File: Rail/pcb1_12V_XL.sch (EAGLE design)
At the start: 114 parts, among them J1 638207222006, J10 638207222006, J11 638207222006, J12 638207222006, J2 638207222006, U1 ESP32-S3-DEVKITC-1-N8R2, U4 TLE9250VSJ, X2 B4P-VH

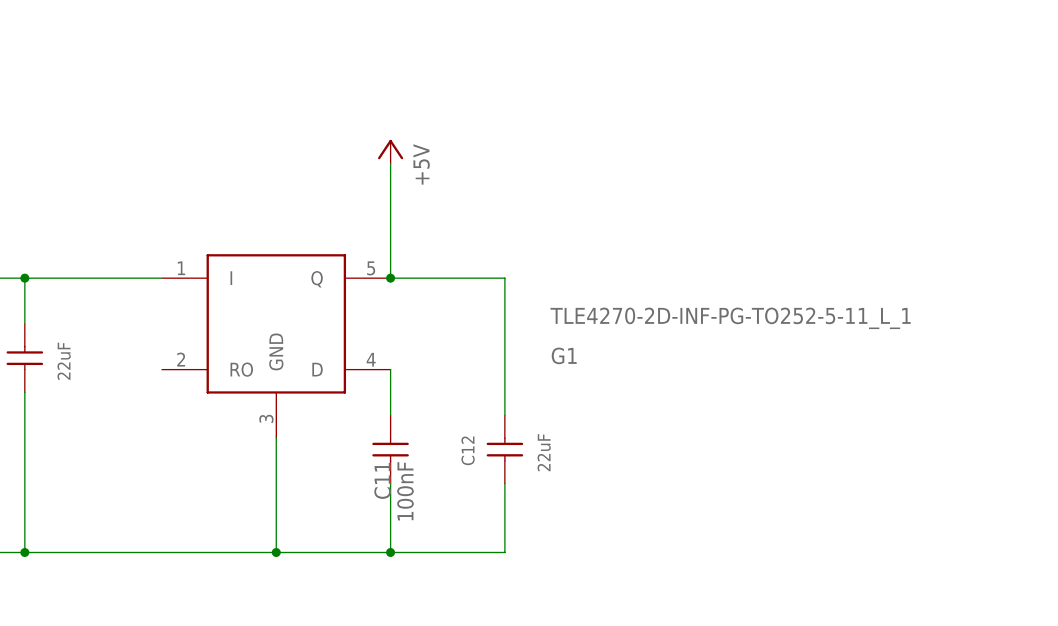
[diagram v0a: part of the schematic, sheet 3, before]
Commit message: Prepare Prouction
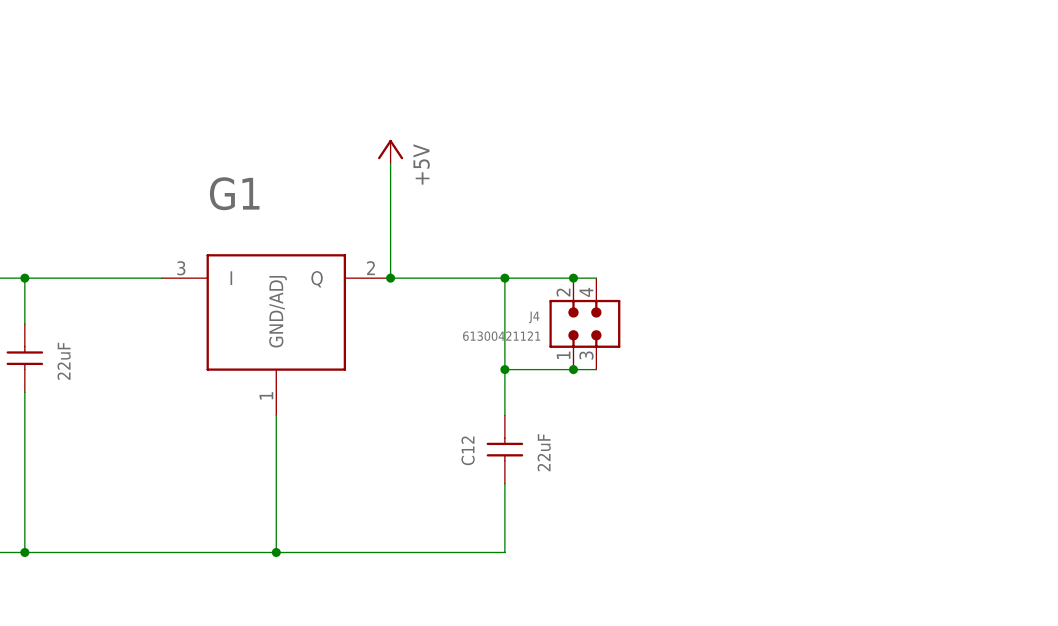
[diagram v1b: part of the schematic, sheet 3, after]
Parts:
- removed C11: 100nF, Wurth_Capacitors_WCAP-CSGP:WCAP-CSGP_0402_885012205037_16V(DC)
- added J4: 61300421121, Wurth_Connectors_WR-PHD:6130XX21121_61300421121
- G1: value TLE4270-2D-INF-PG-TO252-5-11_L_1 -> (none); device INF-PG-TO252-5-11L:TLE4270-2D-INF-PG-TO252-5-11_L_1 -> IFX27001TF V50:IFX27001TF_V50
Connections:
- net N$16 renamed +6V
- removed net N$7: C11.1, G1.D
- net +5V: now also J4.1, J4.2, J4.3, J4.4
- net ECU_GND: now also G1.GND/ADJ; no longer C11.2, G1.GND
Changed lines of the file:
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@@
 <part name="P+4" library="supply1" library_urn="urn:adsk.eagle:library:371" deviceset="+5V" device=""/>
 <part name="C10" library="Wurth_Capacitors_WCAP-CSGP" library_urn="urn:adsk.eagle:library:18488985" deviceset="WCAP-CSGP_1210_H2.5" device="_25V(DC)" package3d_urn="urn:adsk.eagle:package:18489097/2" technology="_885012109014" value="22uF"/>
-<part name="G1" library="INF-PG-TO252-5-11L" deviceset="TLE4270-2D-INF-PG-TO252-5-11_L_1" device=""/>
-<part name="C11" library="Wurth_Capacitors_WCAP-CSGP" library_urn="urn:adsk.eagle:library:18488985" deviceset="WCAP-CSGP_0402" device="_16V(DC)" package3d_urn="urn:adsk.eagle:package:18489133/5" technology="_885012205037" value="100nF"/>
 <part name="C12" library="Wurth_Capacitors_WCAP-CSGP" library_urn="urn:adsk.eagle:library:18488985" deviceset="WCAP-CSGP_0805_H1.25" device="_10V(DC)" package3d_urn="urn:adsk.eagle:package:18489127/2" technology="_885012107011" value="22uF"/>
 <part name="D0" library="Wurth_EMC Components_WE-TVSP" library_urn="urn:adsk.eagle:library:14283044" deviceset="WE-TVSP_DO-214AB_3000W_BI" device="" package3d_urn="urn:adsk.eagle:package:12146529/2" technology="_824551331" value="33V"/>
@@
 <part name="ECU_GND28" library="supply_isobus" deviceset="ECU_GND" device=""/>
 <part name="ECU_GND29" library="supply_isobus" deviceset="ECU_GND" device=""/>
+<part name="G1" library="IFX27001TF V50" deviceset="IFX27001TF_V50" device=""/>
+<part name="J4" library="Wurth_Connectors_WR-PHD" library_urn="urn:adsk.eagle:library:14804658" deviceset="6130XX21121_61300421121" device="" package3d_urn="urn:adsk.eagle:package:14805408/2" value=" 61300421121 "/>
 </parts>
 <sheets>
@@
 <attribute name="VALUE" x="17.775" y="74.575" size="1.4224" layer="96" rot="R90" align="bottom-center"/>
 </instance>
-<instance part="G1" gate="G" x="40.64" y="78.74" smashed="yes">
-<attribute name="NAME" x="71.12" y="74.295" size="1.778" layer="95"/>
-<attribute name="VALUE" x="71.12" y="78.74" size="1.778" layer="96"/>
-</instance>
-<instance part="C11" gate="G$1" x="53.34" y="66.04" smashed="yes" rot="MR270">
-<attribute name="NAME" x="53.34" y="63.5" size="1.778" layer="95" rot="MR270"/>
-<attribute name="VALUE" x="55.88" y="63.5" size="1.778" layer="96" rot="MR270"/>
-</instance>
 <instance part="C12" gate="G$1" x="66.04" y="63.5" smashed="yes" rot="R90">
 <attribute name="NAME" x="62.66" y="64.675" size="1.4224" layer="95" rot="R90" align="bottom-center"/>
@@
 <instance part="ECU_GND28" gate="ECU_GND" x="-25.4" y="119.38" smashed="yes">
 <attribute name="VALUE" x="-27.94" y="116.84" size="1.778" layer="96"/>
+</instance>
+<instance part="G1" gate="G1" x="33.02" y="86.36" smashed="yes">
+<attribute name="NAME" x="33.02" y="91.44" size="3.5306" layer="95" font="vector" ratio="6" rot="SR0"/>
+<attribute name="VALUE" x="33.02" y="63.5" size="3.5306" layer="95" font="vector" ratio="6" rot="SR0"/>
+</instance>
+<instance part="J4" gate="G$1" x="76.2" y="78.74" smashed="yes">
+<attribute name="NAME" x="69.94" y="79.09" size="1.016" layer="95" align="bottom-right"/>
+<attribute name="VALUE" x="70.08" y="76.87" size="1.016" layer="96" align="bottom-right"/>
 </instance>
 </instances>
@@
 <wire x1="12.7" y1="78.74" x2="12.7" y2="83.82" width="0.1524" layer="91"/>
 <junction x="12.7" y="83.82"/>
-<pinref part="G1" gate="G" pin="I"/>
 <pinref part="D5" gate="G$1" pin="2"/>
 <junction x="-10.16" y="83.82"/>
 <pinref part="ECU_PWR2" gate="ECU_PWR" pin="ECU_PWR"/>
+<pinref part="G1" gate="G1" pin="I"/>
 </segment>
 <segment>
@@
 </segment>
 </net>
-<net name="N$7" class="0">
-<segment>
-<pinref part="G1" gate="G" pin="D"/>
-<pinref part="C11" gate="G$1" pin="1"/>
-<wire x1="53.34" y1="73.66" x2="53.34" y2="68.58" width="0.1524" layer="91"/>
-</segment>
-</net>
 <net name="ECU_GND" class="1">
 <segment>
 <pinref part="C12" gate="G$1" pin="1"/>
 <wire x1="66.04" y1="53.34" x2="66.04" y2="60.96" width="0.1524" layer="91"/>
-<pinref part="C11" gate="G$1" pin="2"/>
-<wire x1="53.34" y1="60.96" x2="53.34" y2="53.34" width="0.1524" layer="91"/>
-<wire x1="66.04" y1="53.34" x2="53.34" y2="53.34" width="0.1524" layer="91"/>
-<pinref part="G1" gate="G" pin="GND"/>
-<wire x1="40.64" y1="53.34" x2="40.64" y2="66.04" width="0.1524" layer="91"/>
-<wire x1="53.34" y1="53.34" x2="40.64" y2="53.34" width="0.1524" layer="91"/>
-<junction x="53.34" y="53.34"/>
+<wire x1="40.64" y1="53.34" x2="40.64" y2="68.58" width="0.1524" layer="91"/>
+<wire x1="66.04" y1="53.34" x2="40.64" y2="53.34" width="0.1524" layer="91"/>
 <pinref part="D5" gate="G$1" pin="1"/>
 <wire x1="40.64" y1="53.34" x2="12.7" y2="53.34" width="0.1524" layer="91"/>
@@
 <junction x="12.7" y="53.34"/>
 <pinref part="ECU_GND2" gate="ECU_GND" pin="ECU_GND"/>
+<pinref part="G1" gate="G1" pin="GND/ADJ"/>
 </segment>
 <segment>
@@
 <segment>
 <pinref part="P+4" gate="1" pin="+5V"/>
-<pinref part="G1" gate="G" pin="Q"/>
 <wire x1="53.34" y1="96.52" x2="53.34" y2="83.82" width="0.1524" layer="91"/>
 <pinref part="C12" gate="G$1" pin="2"/>
 <wire x1="53.34" y1="83.82" x2="66.04" y2="83.82" width="0.1524" layer="91"/>
-<wire x1="66.04" y1="83.82" x2="66.04" y2="68.58" width="0.1524" layer="91"/>
+<wire x1="66.04" y1="83.82" x2="66.04" y2="73.66" width="0.1524" layer="91"/>
 <junction x="53.34" y="83.82"/>
+<pinref part="G1" gate="G1" pin="Q"/>
+<pinref part="J4" gate="G$1" pin="4"/>
+<pinref part="J4" gate="G$1" pin="2"/>
+<wire x1="66.04" y1="73.66" x2="66.04" y2="68.58" width="0.1524" layer="91"/>
+<wire x1="76.2" y1="83.82" x2="73.66" y2="83.82" width="0.1524" layer="91"/>
+<wire x1="73.66" y1="83.82" x2="66.04" y2="83.82" width="0.1524" layer="91"/>
+<junction x="73.66" y="83.82"/>
+<junction x="66.04" y="83.82"/>
+<pinref part="J4" gate="G$1" pin="3"/>
+<pinref part="J4" gate="G$1" pin="1"/>
+<wire x1="76.2" y1="73.66" x2="73.66" y2="73.66" width="0.1524" layer="91"/>
+<wire x1="73.66" y1="73.66" x2="66.04" y2="73.66" width="0.1524" layer="91"/>
+<junction x="73.66" y="73.66"/>
+<junction x="66.04" y="73.66"/>
 </segment>
 </net>
@@
 </segment>
 </net>
-<net name="N$16" class="1">
+<net name="+6V" class="1">
 <segment>
 <wire x1="157.48" y1="129.54" x2="157.48" y2="139.7" width="0.1524" layer="91"/>

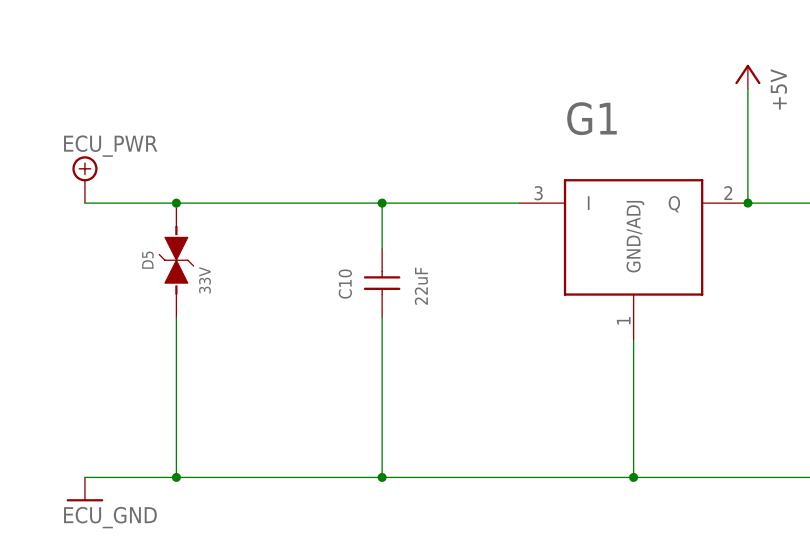
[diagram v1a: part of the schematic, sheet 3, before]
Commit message: verpolschutz.
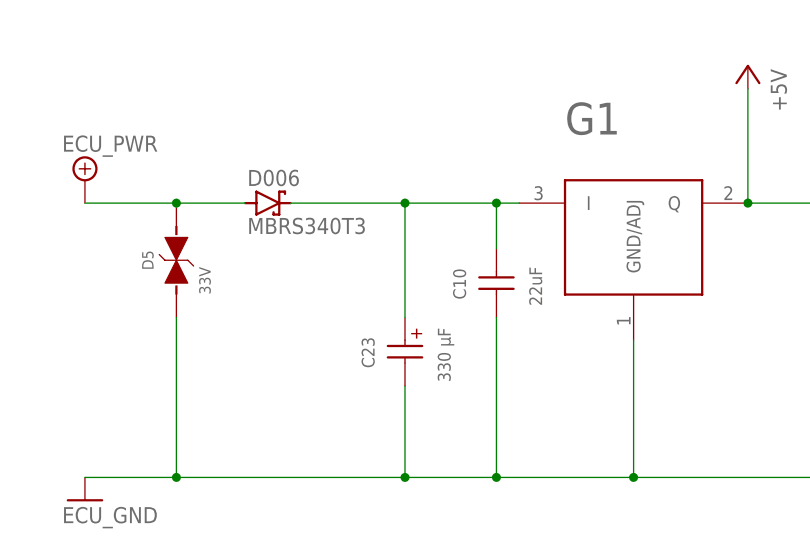
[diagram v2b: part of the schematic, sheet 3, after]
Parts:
- added C23: 330 µF, Wurth_Capacitors_WCAP-ASLI:WCAP-ASLI_12.5X14_865080662019
- added D006: MBRS340T3, fliegl-elektronik:MBRS340T3
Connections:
- new net N$3: C10.2, C23.+, D006.C, G1.I
- net ECU_GND: now also C23.-
- net ECU_PWR: now also D006.A; no longer C10.2, G1.I
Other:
- moved on the sheet: C10
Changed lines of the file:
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@@
 <part name="G1" library="IFX27001TF V50" deviceset="IFX27001TF_V50" device=""/>
 <part name="J4" library="Wurth_Connectors_WR-PHD" library_urn="urn:adsk.eagle:library:14804658" deviceset="6130XX21121_61300421121" device="" package3d_urn="urn:adsk.eagle:package:14805408/2" value=" 61300421121 "/>
+<part name="D006" library="fliegl-elektronik" deviceset="MBRS3*0T3" device="" technology="4"/>
+<part name="C23" library="Wurth_Capacitors_WCAP-ASLI" library_urn="urn:adsk.eagle:library:18353966" deviceset="WCAP-ASLI_12.5X14" device="" package3d_urn="urn:adsk.eagle:package:18353982/3" technology="_865080662019" value="330  µF "/>
 </parts>
 <sheets>
@@
 <attribute name="VALUE" x="55.88" y="93.98" size="1.778" layer="96" rot="MR90"/>
 </instance>
-<instance part="C10" gate="G$1" x="12.7" y="73.66" smashed="yes" rot="R90">
-<attribute name="NAME" x="9.32" y="74.835" size="1.4224" layer="95" rot="R90" align="bottom-center"/>
-<attribute name="VALUE" x="17.775" y="74.575" size="1.4224" layer="96" rot="R90" align="bottom-center"/>
+<instance part="C10" gate="G$1" x="25.4" y="73.66" smashed="yes" rot="R90">
+<attribute name="NAME" x="22.02" y="74.835" size="1.4224" layer="95" rot="R90" align="bottom-center"/>
+<attribute name="VALUE" x="30.475" y="74.575" size="1.4224" layer="96" rot="R90" align="bottom-center"/>
 </instance>
 <instance part="C12" gate="G$1" x="66.04" y="63.5" smashed="yes" rot="R90">
@@
 <attribute name="NAME" x="69.94" y="79.09" size="1.016" layer="95" align="bottom-right"/>
 <attribute name="VALUE" x="70.08" y="76.87" size="1.016" layer="96" align="bottom-right"/>
+</instance>
+<instance part="D006" gate="G$1" x="0" y="83.82" smashed="yes">
+<attribute name="NAME" x="-2.286" y="85.725" size="1.778" layer="95"/>
+<attribute name="VALUE" x="-2.286" y="80.391" size="1.778" layer="96"/>
+</instance>
+<instance part="C23" gate="G$1" x="15.24" y="66.04" smashed="yes" rot="R90">
+<attribute name="NAME" x="11.86" y="67.215" size="1.4224" layer="95" rot="R90" align="bottom-center"/>
+<attribute name="VALUE" x="20.315" y="66.955" size="1.4224" layer="96" rot="R90" align="bottom-center"/>
 </instance>
 </instances>
@@
 <net name="ECU_PWR" class="0">
 <segment>
-<pinref part="C10" gate="G$1" pin="2"/>
-<wire x1="-20.32" y1="83.82" x2="-10.16" y2="83.82" width="0.1524" layer="91"/>
-<wire x1="-10.16" y1="83.82" x2="12.7" y2="83.82" width="0.1524" layer="91"/>
-<wire x1="12.7" y1="83.82" x2="27.94" y2="83.82" width="0.1524" layer="91"/>
-<wire x1="12.7" y1="78.74" x2="12.7" y2="83.82" width="0.1524" layer="91"/>
-<junction x="12.7" y="83.82"/>
 <pinref part="D5" gate="G$1" pin="2"/>
 <junction x="-10.16" y="83.82"/>
+<wire x1="-10.16" y1="83.82" x2="-2.54" y2="83.82" width="0.1524" layer="91"/>
+<wire x1="-20.32" y1="83.82" x2="-10.16" y2="83.82" width="0.1524" layer="91"/>
 <pinref part="ECU_PWR2" gate="ECU_PWR" pin="ECU_PWR"/>
-<pinref part="G1" gate="G1" pin="I"/>
+<pinref part="D006" gate="G$1" pin="A"/>
 </segment>
 <segment>
@@
 <wire x1="66.04" y1="53.34" x2="40.64" y2="53.34" width="0.1524" layer="91"/>
 <pinref part="D5" gate="G$1" pin="1"/>
-<wire x1="40.64" y1="53.34" x2="12.7" y2="53.34" width="0.1524" layer="91"/>
-<wire x1="12.7" y1="53.34" x2="-10.16" y2="53.34" width="0.1524" layer="91"/>
+<wire x1="40.64" y1="53.34" x2="25.4" y2="53.34" width="0.1524" layer="91"/>
+<wire x1="25.4" y1="53.34" x2="15.24" y2="53.34" width="0.1524" layer="91"/>
+<wire x1="15.24" y1="53.34" x2="-10.16" y2="53.34" width="0.1524" layer="91"/>
 <wire x1="-10.16" y1="53.34" x2="-10.16" y2="71.12" width="0.1524" layer="91"/>
 <junction x="40.64" y="53.34"/>
@@
 <junction x="-10.16" y="53.34"/>
 <pinref part="C10" gate="G$1" pin="1"/>
-<wire x1="12.7" y1="71.12" x2="12.7" y2="53.34" width="0.1524" layer="91"/>
-<junction x="12.7" y="53.34"/>
+<wire x1="25.4" y1="71.12" x2="25.4" y2="53.34" width="0.1524" layer="91"/>
+<junction x="25.4" y="53.34"/>
 <pinref part="ECU_GND2" gate="ECU_GND" pin="ECU_GND"/>
 <pinref part="G1" gate="G1" pin="GND/ADJ"/>
+<wire x1="15.24" y1="63.5" x2="15.24" y2="53.34" width="0.1524" layer="91"/>
+<junction x="15.24" y="53.34"/>
+<pinref part="C23" gate="G$1" pin="-"/>
 </segment>
 <segment>
@@
 </segment>
 </net>
+<net name="N$3" class="0">
+<segment>
+<pinref part="C10" gate="G$1" pin="2"/>
+<wire x1="25.4" y1="83.82" x2="27.94" y2="83.82" width="0.1524" layer="91"/>
+<wire x1="25.4" y1="78.74" x2="25.4" y2="83.82" width="0.1524" layer="91"/>
+<junction x="25.4" y="83.82"/>
+<pinref part="G1" gate="G1" pin="I"/>
+<wire x1="2.54" y1="83.82" x2="15.24" y2="83.82" width="0.1524" layer="91"/>
+<pinref part="D006" gate="G$1" pin="C"/>
+<wire x1="15.24" y1="83.82" x2="25.4" y2="83.82" width="0.1524" layer="91"/>
+<wire x1="15.24" y1="71.12" x2="15.24" y2="83.82" width="0.1524" layer="91"/>
+<junction x="15.24" y="83.82"/>
+<pinref part="C23" gate="G$1" pin="+"/>
+</segment>
+</net>
